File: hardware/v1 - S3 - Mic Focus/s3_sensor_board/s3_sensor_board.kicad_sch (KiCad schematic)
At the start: 7 parts, among them J101 Conn_01x02

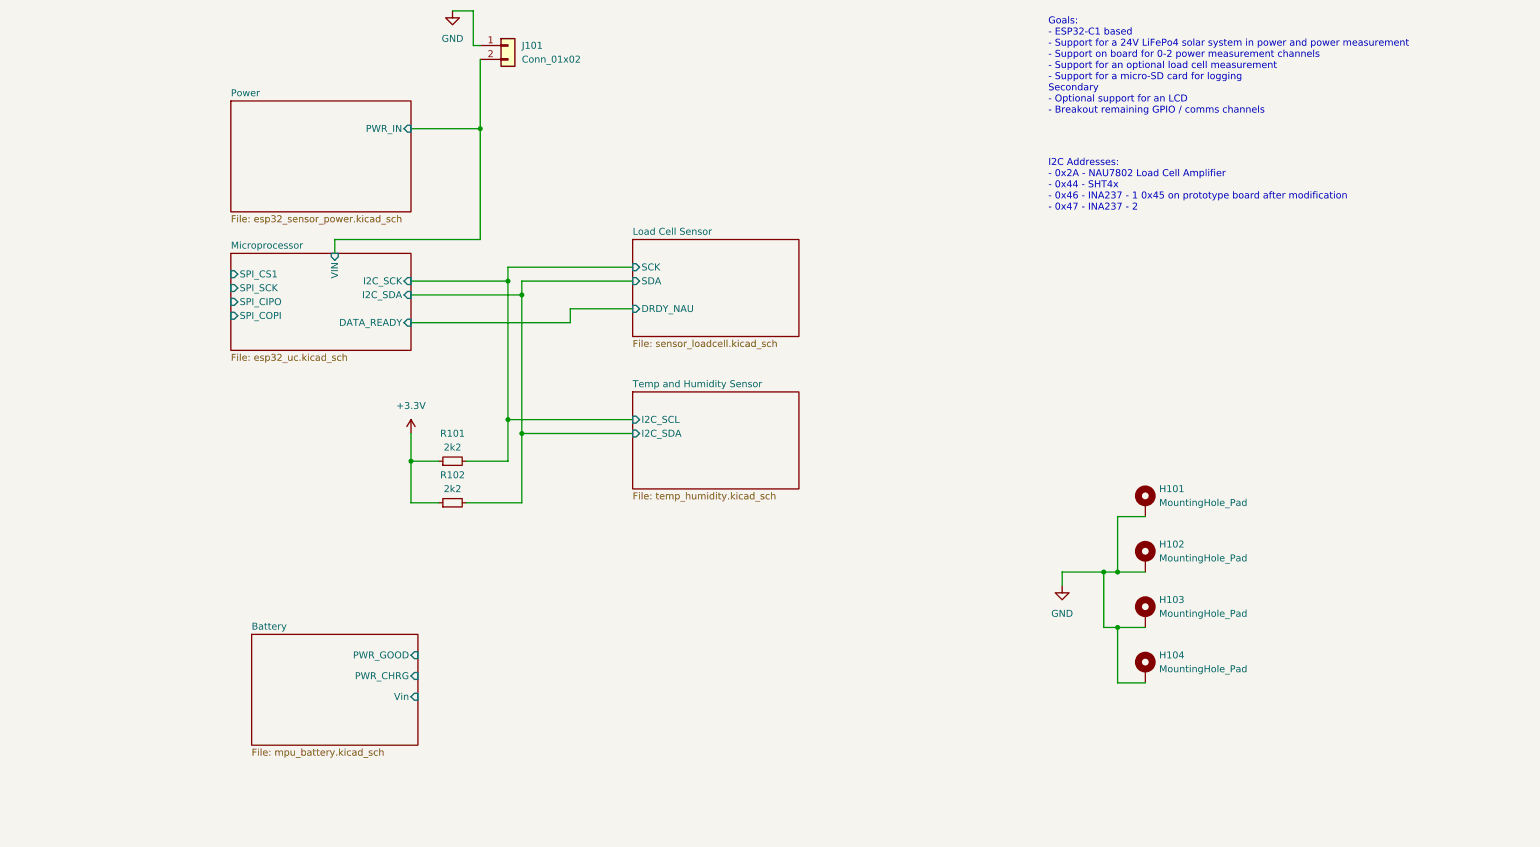
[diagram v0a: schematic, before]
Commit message: WIP
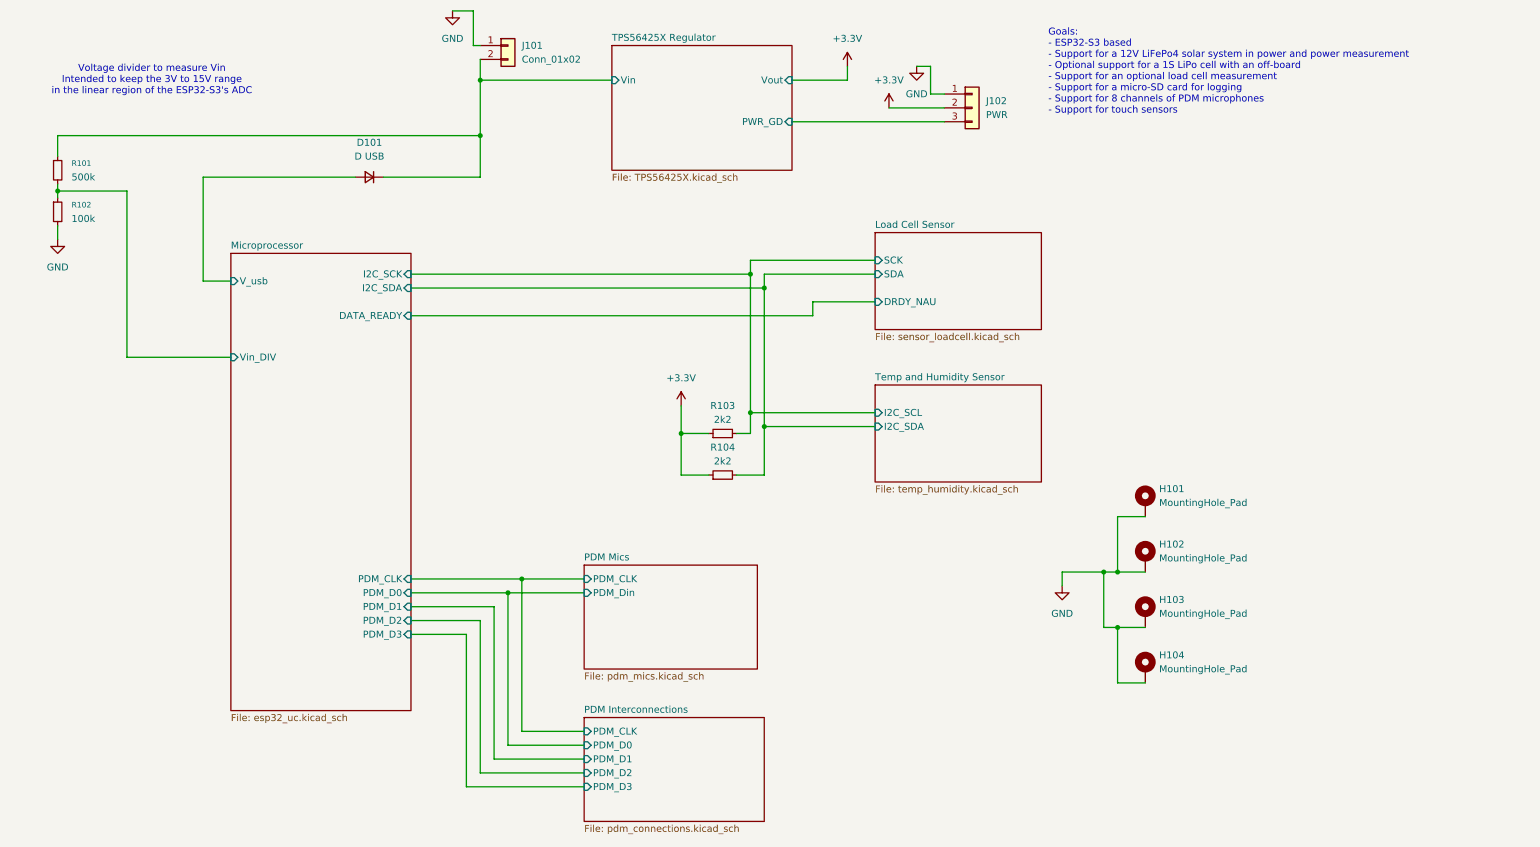
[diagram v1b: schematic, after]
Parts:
- added D101: D USB, Diode_SMD:D_SOD-123, symbol Device:D_Small
- added J102: PWR, Connector_PinHeader_2.54mm:PinHeader_1x03_P2.54mm_Vertical, symbol Connector_Generic:Conn_01x03
- added R101: 500k, Resistor_SMD:R_0603_1608Metric, symbol Device:R_Small
- added R102: 100k, Resistor_SMD:R_0603_1608Metric, symbol Device:R_Small
- J101: footprint Connector_Phoenix_MSTB:PhoenixContact_MSTBA_2,5_2-G-5,08_1x02_P5.08mm_Horizontal -> Connector_PinHeader_2.54mm:PinHeader_1x02_P2.54mm_Vertical
- renumbered R101 to R103, R102 to R104
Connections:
- net +3.3V: now also J102.2 (Pin_2)
- net GND: now also J102.1 (Pin_1), R102.2
- net Microprocessor/VIN renamed TPS56425X Regulator/Vin
- net TPS56425X Regulator/Vin: now also D101.1 (K), R101.1
- new net Microprocessor/V_usb: D101.2 (A)
- new net Microprocessor/Vin_DIV: R101.2, R102.1
- new net TPS56425X Regulator/PWR_GD: J102.3 (Pin_3)
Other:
- removed sheet Battery
- removed sheet Power
- added sheet PDM Interconnections (pdm_connections.kicad_sch)
- added sheet PDM Mics (pdm_mics.kicad_sch)
- added sheet TPS56425X Regulator (TPS56425X.kicad_sch)
- sheet Microprocessor ports: added PDM_CLK, PDM_D0, PDM_D1, PDM_D2, PDM_D3, V_usb, Vin_DIV; removed SPI_CIPO, SPI_COPI, SPI_CS1, SPI_SCK, VIN
- note added: "Goals: - ESP32-S3 based - Support for a 12V LiFePo4 solar system in power and power measurement - Optional support for a 1S LiPo cell with an off-board - Support for an optional load cell measurement - Support for a micro-SD card for logging - Support for 8 channels of PDM microphones - Support for touch sensors"
- note added: "Voltage divider to measure Vin Intended to keep the 3V to 15V range in the linear region of the ESP32-S3's ADC"
- note removed: "Goals: - ESP32-C1 based - Support for a 24V LiFePo4 solar system in power and power measurement - Support on board for 0-2 power measurement channels - Support for an optional load cell measurement - Support for a micro-SD card for logging Secondary - Optional support for an LCD - Breakout remaining GPIO / comms channels"
- note removed: "I2C Addresses: - 0x2A - NAU7802 Load Cell Amplifier - 0x44 - SHT4x - 0x46 - INA237 - 1 0x45 on prototype board after modification - 0x47 - INA237 - 2"
- moved on the sheet: R103, R104
